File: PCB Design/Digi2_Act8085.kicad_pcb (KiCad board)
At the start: 2 copper layers, 27 parts, among them U1 8085A, U10 8255, U2 Barrel_Jack, U3 L7805, U4 2764, U5 CY6264, U6 74LS373, U7 74LS138, U8 8255, U9 8255, Y1 3MHz

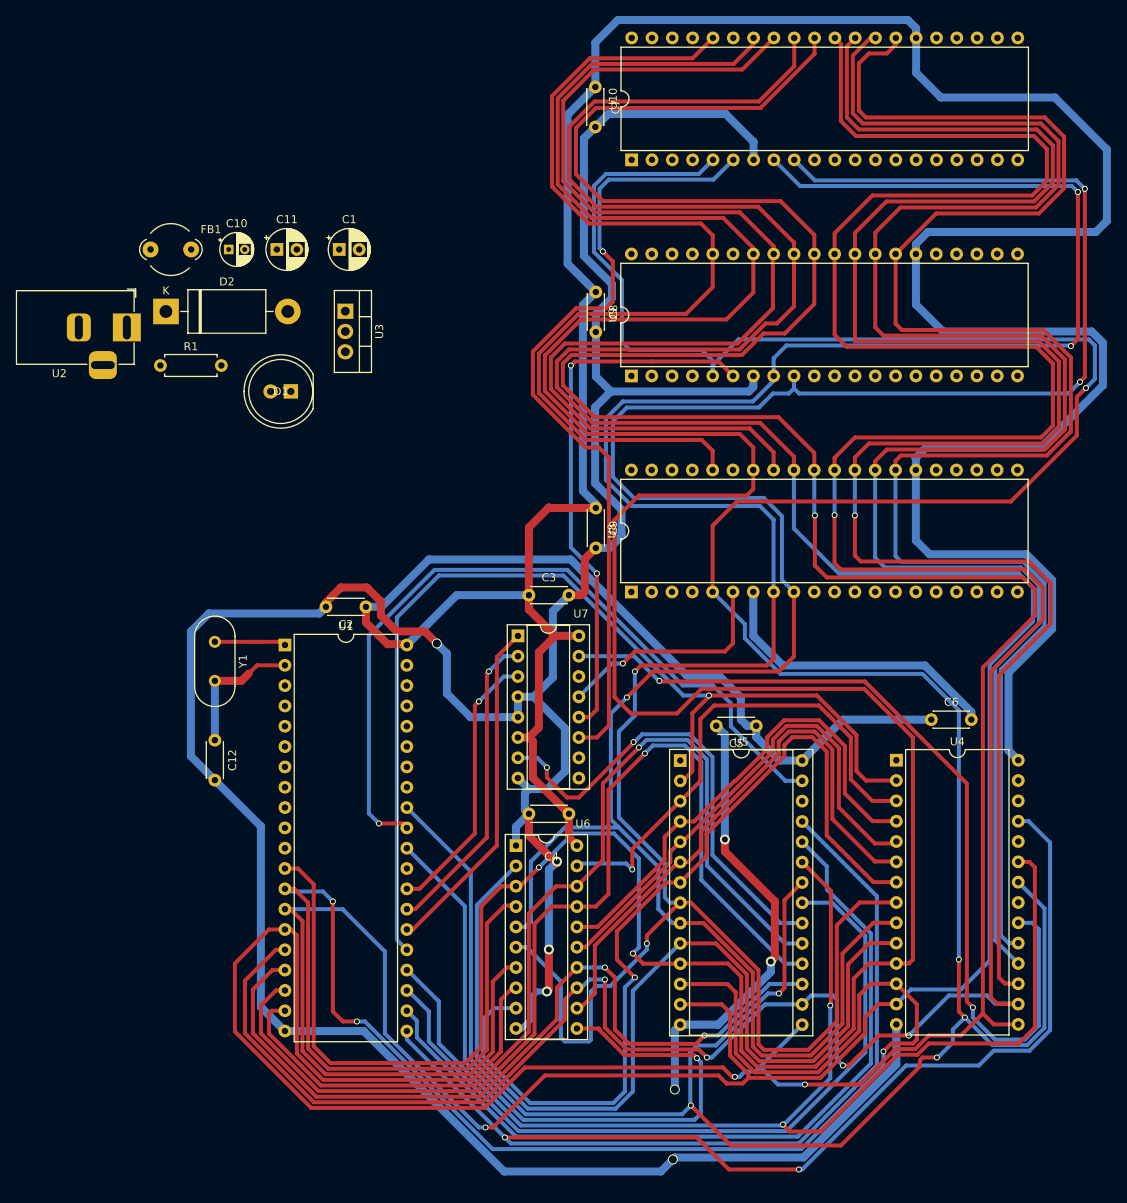
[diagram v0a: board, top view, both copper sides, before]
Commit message: newwwwwwwwwwwwwwwwww
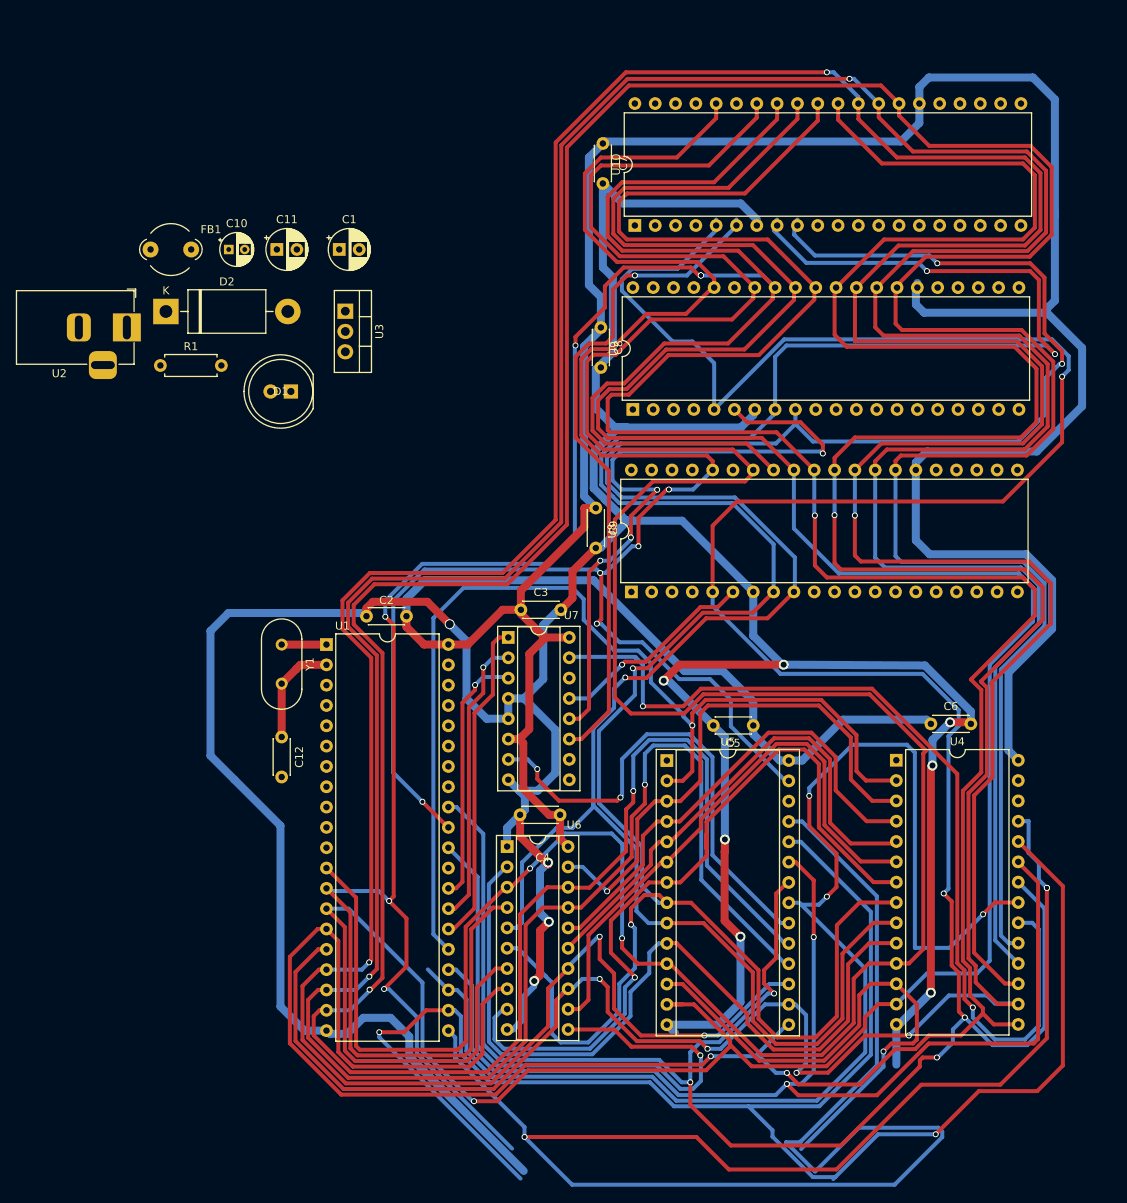
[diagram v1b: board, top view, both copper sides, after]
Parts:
- moved C12 8.36 mm to (61.9, 108.4)
- moved Y1 8.36 mm to (61.9, 96.9)
- moved U10 8.21 mm to (106.0, 44.5)
- moved C7 7.12 mm to (102.0, 34.2)
- moved C2 5.20 mm to (77.5, 93.3)
- moved U1 5.20 mm to (67.5, 96.9)
- moved C8 4.48 mm to (101.8, 57.2)
- moved U9 4.20 mm to (105.8, 67.5)
- moved C3 2.09 mm to (91.8, 92.5)
- moved U5 1.67 mm to (110.0, 111.4)
- moved U7 1.22 mm to (90.2, 96.0)
- moved U6 1.11 mm to (90.0, 122.1)
- moved C4 1.11 mm to (96.7, 118.2)
- moved C6 0.53 mm to (143.0, 106.8)
- moved C5 0.38 mm to (120.8, 107.0)
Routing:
- net /Memory and Peripheral Inteface/AD5: track 340.1 -> 489.4 mm, vias 3 -> 5
- net /Memory and Peripheral Inteface/AD7: track 340.6 -> 487.0 mm, vias 1 -> 2
- net /Memory and Peripheral Inteface/AD6: track 356.4 -> 500.4 mm, vias 1 -> 3
- net /Memory and Peripheral Inteface/A9: track 100.8 -> 210.2 mm, vias 0 -> 2
- net /Memory and Peripheral Inteface/A10: track 95.0 -> 166.2 mm, vias 0 -> 3
- net +5V: track 464.5 -> 409.1 mm
- net /Memory and Peripheral Inteface/AD2: track 430.6 -> 379.8 mm
- net /Memory and Peripheral Inteface/AD3: track 441.7 -> 395.9 mm
- net /Memory and Peripheral Inteface/A8: track 209.1 -> 253.5 mm, vias 2 -> 3
- net /Memory and Peripheral Inteface/AD0: track 408.2 -> 366.3 mm
- net /Memory and Peripheral Inteface/AD1: track 369.9 -> 409.5 mm, vias 3 -> 7
- net /Memory and Peripheral Inteface/AD4: track 391.5 -> 368.8 mm
- net /Memory and Peripheral Inteface/~{RD}: track 427.2 -> 404.6 mm
- net /Memory and Peripheral Inteface/A0: track 119.2 -> 99.5 mm
- net /Memory and Peripheral Inteface/~{Y4}: track 101.6 -> 83.6 mm
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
